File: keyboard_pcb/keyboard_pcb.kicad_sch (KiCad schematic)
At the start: 190 parts, among them SW1 SW_Push, U1 ATmega32U4-A, Y1 16MHz

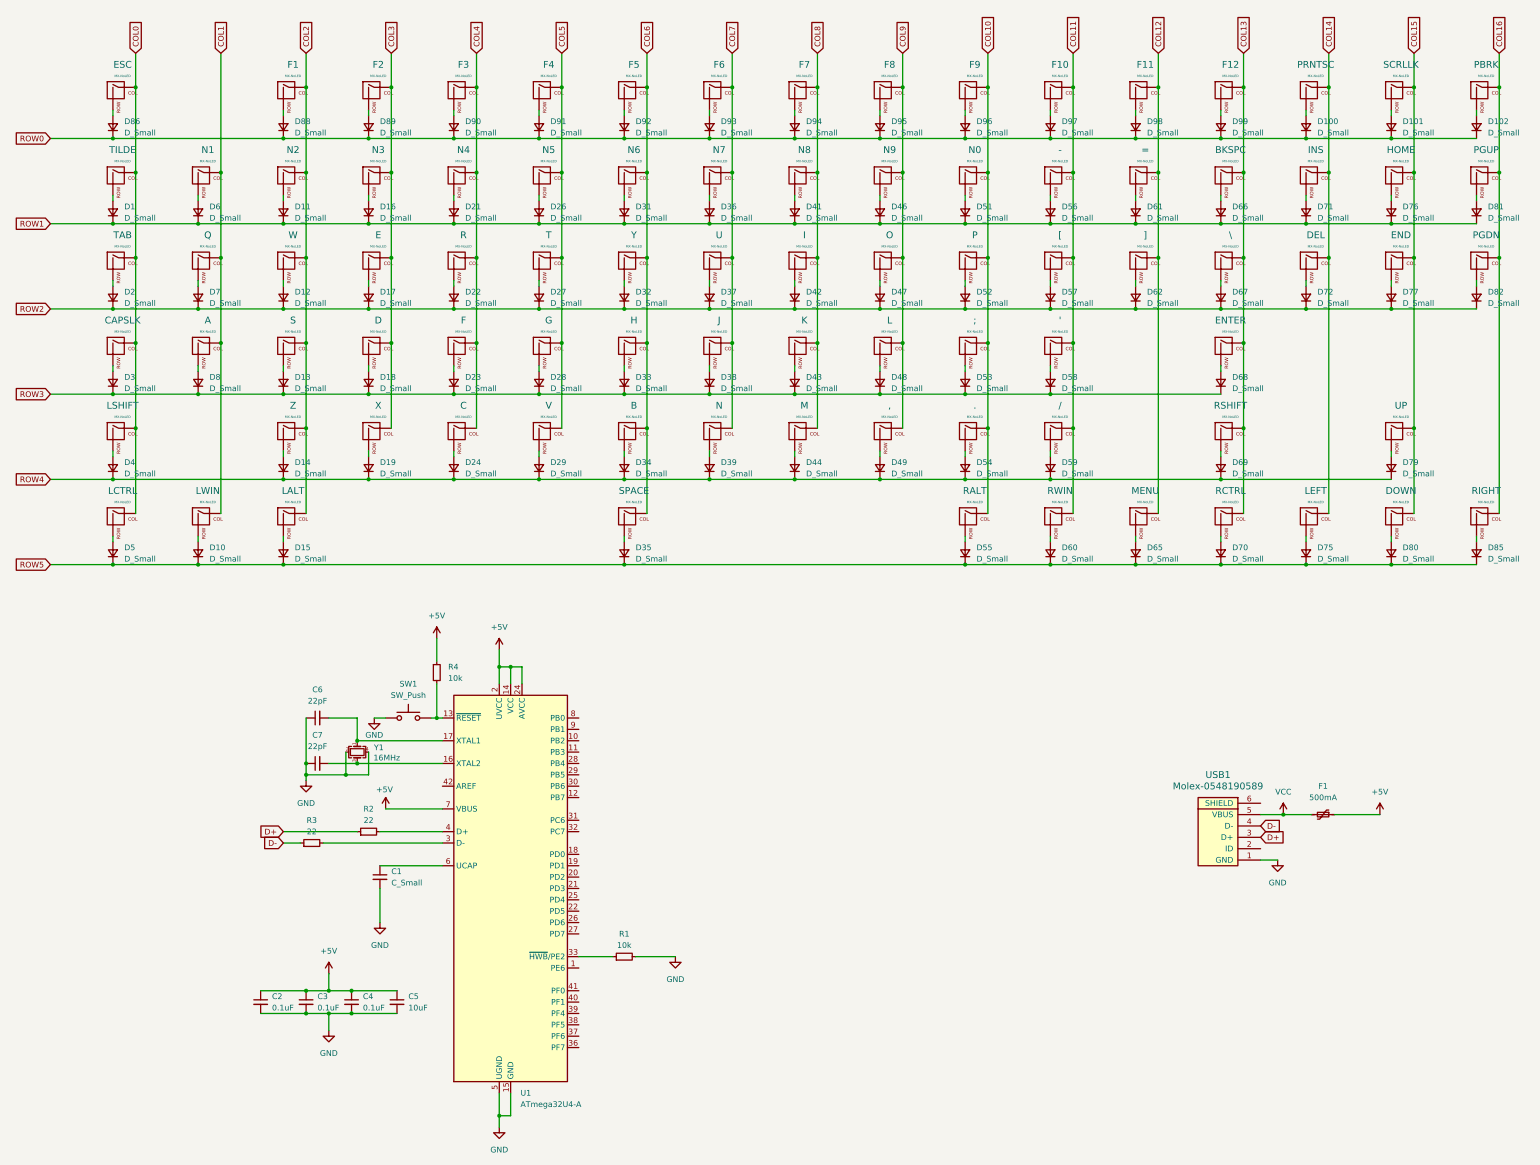
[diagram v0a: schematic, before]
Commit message: Complete electronic schematic
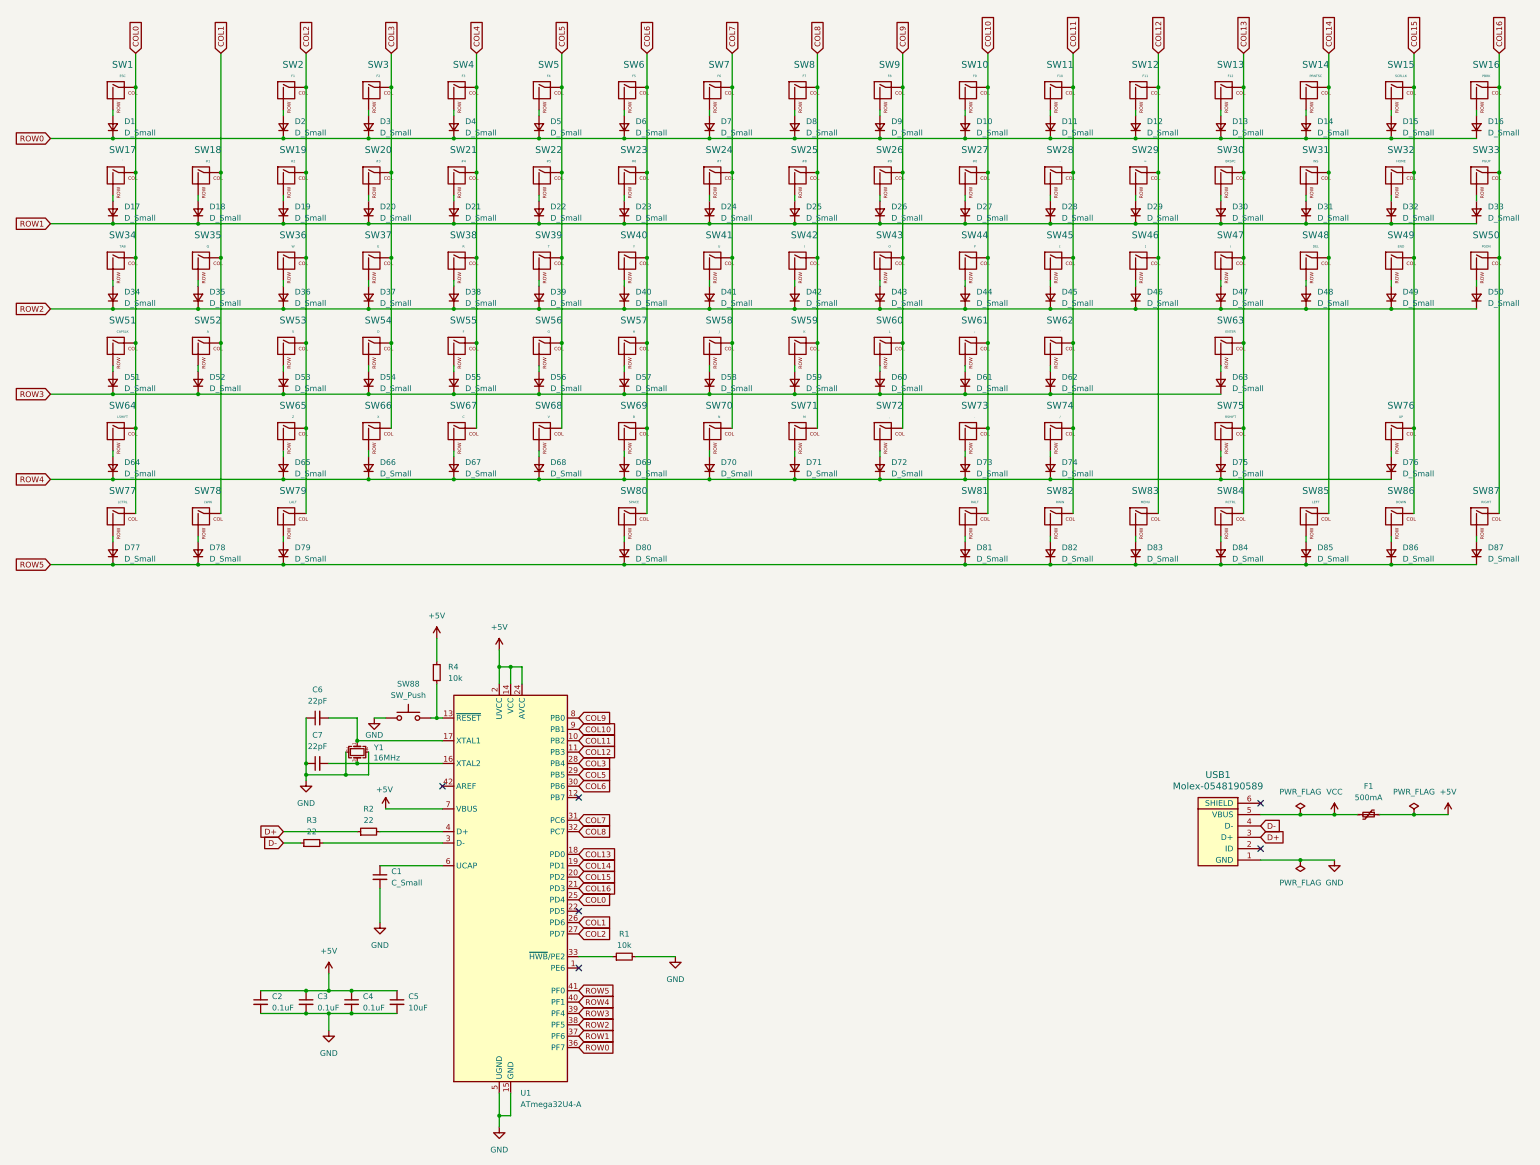
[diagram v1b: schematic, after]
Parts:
- SW1: renamed from ESC; value MX-NoLED -> ESC
- SW10: renamed from F9; value MX-NoLED -> F9
- SW11: renamed from F10; value MX-NoLED -> F10
- SW12: renamed from F11; value MX-NoLED -> F11
- SW13: renamed from F12; value MX-NoLED -> F12
- SW14: renamed from PRNTSC; value MX-NoLED -> PRNTSC
- SW15: renamed from SCRLLK; value MX-NoLED -> SCRLLK
- SW16: renamed from PBRK; value MX-NoLED -> PBRK
- SW17: renamed from TILDE; value MX-NoLED -> `
- SW18: renamed from N1; value MX-NoLED -> #1
- SW19: renamed from N2; value MX-NoLED -> #2
- SW2: renamed from F1; value MX-NoLED -> F1
- SW20: renamed from N3; value MX-NoLED -> #3
- SW21: renamed from N4; value MX-NoLED -> #4
- SW22: renamed from N5; value MX-NoLED -> #5
- SW23: renamed from N6; value MX-NoLED -> #6
- SW24: renamed from N7; value MX-NoLED -> #7
- SW25: renamed from N8; value MX-NoLED -> #8
- SW26: renamed from N9; value MX-NoLED -> #9
- SW27: renamed from N0; value MX-NoLED -> #0
- SW28: renamed from -; value MX-NoLED -> -
- SW29: renamed from =; value MX-NoLED -> =
- SW3: renamed from F2; value MX-NoLED -> F2
- SW30: renamed from BKSPC; value MX-NoLED -> BKSPC
- SW31: renamed from INS; value MX-NoLED -> INS
- SW32: renamed from HOME; value MX-NoLED -> HOME
- SW33: renamed from PGUP; value MX-NoLED -> PGUP
- SW34: renamed from TAB; value MX-NoLED -> TAB
- SW35: renamed from Q; value MX-NoLED -> Q
- SW36: renamed from W; value MX-NoLED -> W
- SW37: renamed from E; value MX-NoLED -> E
- SW38: renamed from R; value MX-NoLED -> R
- SW39: renamed from T; value MX-NoLED -> T
- SW4: renamed from F3; value MX-NoLED -> F3
- SW40: renamed from Y; value MX-NoLED -> Y
- SW41: renamed from U; value MX-NoLED -> U
- SW42: renamed from I; value MX-NoLED -> I
- SW43: renamed from O; value MX-NoLED -> O
- SW44: renamed from P; value MX-NoLED -> P
- SW45: renamed from [; value MX-NoLED -> [
- SW46: renamed from ]; value MX-NoLED -> ]
- SW47: renamed from \; value MX-NoLED -> \
- SW48: renamed from DEL; value MX-NoLED -> DEL
- SW49: renamed from END; value MX-NoLED -> END
- SW5: renamed from F4; value MX-NoLED -> F4
- SW50: renamed from PGDN; value MX-NoLED -> PGDN
- SW51: renamed from CAPSLK; value MX-NoLED -> CAPSLK
- SW52: renamed from A; value MX-NoLED -> A
- SW53: renamed from S; value MX-NoLED -> S
- SW54: renamed from D; value MX-NoLED -> D
- SW55: renamed from F; value MX-NoLED -> F
- SW56: renamed from G; value MX-NoLED -> G
- SW57: renamed from H; value MX-NoLED -> H
- SW58: renamed from J; value MX-NoLED -> J
- SW59: renamed from K; value MX-NoLED -> K
- SW6: renamed from F5; value MX-NoLED -> F5
- SW60: renamed from L; value MX-NoLED -> L
- SW61: renamed from ;; value MX-NoLED -> ;
- SW62: renamed from '; value MX-NoLED -> '
- SW63: renamed from ENTER; value MX-NoLED -> ENTER
- SW64: renamed from LSHIFT; value MX-NoLED -> LSHIFT
- SW65: renamed from Z; value MX-NoLED -> Z
- SW66: renamed from X; value MX-NoLED -> X
- SW67: renamed from C; value MX-NoLED -> C
- SW68: renamed from V; value MX-NoLED -> V
- SW69: renamed from B; value MX-NoLED -> B
- SW7: renamed from F6; value MX-NoLED -> F6
- SW70: renamed from N; value MX-NoLED -> N
- SW71: renamed from M; value MX-NoLED -> M
- SW72: renamed from ,; value MX-NoLED -> ,
- SW73: renamed from .; value MX-NoLED -> .
- SW74: renamed from /; value MX-NoLED -> /
- SW75: renamed from RSHIFT; value MX-NoLED -> RSHIFT
- SW76: renamed from UP; value MX-NoLED -> UP
- SW77: renamed from LCTRL; value MX-NoLED -> LCTRL
- SW78: renamed from LWIN; value MX-NoLED -> LWIN
- SW79: renamed from LALT; value MX-NoLED -> LALT
- SW8: renamed from F7; value MX-NoLED -> F7
- SW80: renamed from SPACE; value MX-NoLED -> SPACE
- SW81: renamed from RALT; value MX-NoLED -> RALT
- SW82: renamed from RWIN; value MX-NoLED -> RWIN
- SW83: renamed from MENU; value MX-NoLED -> MENU
- SW84: renamed from RCTRL; value MX-NoLED -> RCTRL
- SW85: renamed from LEFT; value MX-NoLED -> LEFT
- SW86: renamed from DOWN; value MX-NoLED -> DOWN
- SW87: renamed from RIGHT; value MX-NoLED -> RIGHT
- SW9: renamed from F8; value MX-NoLED -> F8
- renumbered D86 to D1, D96 to D10, D97 to D11, D98 to D12, D99 to D13, D100 to D14, D101 to D15, D102 to D16, D1 to D17, D6 to D18, D11 to D19, D88 to D2, D16 to D20, D26 to D22, D31 to D23, D36 to D24, D41 to D25, D46 to D26, D51 to D27, D56 to D28, D61 to D29, D89 to D3, D66 to D30, D71 to D31, D76 to D32, D81 to D33, D2 to D34, D7 to D35, D12 to D36, D17 to D37, D22 to D38, D27 to D39, D90 to D4, D32 to D40, D37 to D41, D47 to D43, D52 to D44, D57 to D45, D62 to D46, D67 to D47, D72 to D48, D77 to D49, D91 to D5, D82 to D50, D3 to D51, D8 to D52, D13 to D53, D18 to D54, D23 to D55, D28 to D56, D33 to D57, D38 to D58, D43 to D59, D92 to D6, D48 to D60, D53 to D61, D58 to D62, D68 to D63, D4 to D64, D14 to D65, D19 to D66, D24 to D67, D29 to D68, D34 to D69, D93 to D7, D39 to D70, D44 to D71, D49 to D72, D54 to D73, D59 to D74, D69 to D75, D79 to D76, D5 to D77, D10 to D78, D15 to D79, D94 to D8, D35 to D80, D55 to D81, D60 to D82, D65 to D83, D70 to D84, D75 to D85, D80 to D86, D85 to D87, D95 to D9, SW1 to SW88
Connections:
- net COL0: now also U1.25 (PD4)
- net COL1: now also U1.26 (PD6)
- net COL10: now also U1.9 (PB1)
- net COL11: now also U1.10 (PB2)
- net COL12: now also U1.11 (PB3)
- net COL13: now also U1.18 (PD0)
- net COL14: now also U1.19 (PD1)
- net COL15: now also U1.20 (PD2)
- net COL16: now also U1.21 (PD3)
- net COL2: now also U1.27 (PD7)
- net COL3: now also U1.28 (PB4)
- net COL5: now also U1.29 (PB5)
- net COL6: now also U1.30 (PB6)
- net COL7: now also U1.31 (PC6)
- net COL8: now also U1.32 (PC7)
- net COL9: now also U1.8 (PB0)
- net ROW0: now also U1.36 (PF7)
- net ROW1: now also U1.37 (PF6)
- net ROW2: now also U1.38 (PF5)
- net ROW3: now also U1.39 (PF4)
- net ROW4: now also U1.40 (PF1)
- net ROW5: now also U1.41 (PF0)
- no-connect marks 0 -> 6
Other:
- moved on the sheet: F1
